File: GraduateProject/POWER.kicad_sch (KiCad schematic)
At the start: 24 parts, among them J2 Conn_01x04_Pin, U1 TLP181GB-S, U2 78L05G-AB3-R, U3 78L05G-AB3-R, U4 26V-15V L78L15ABUTR

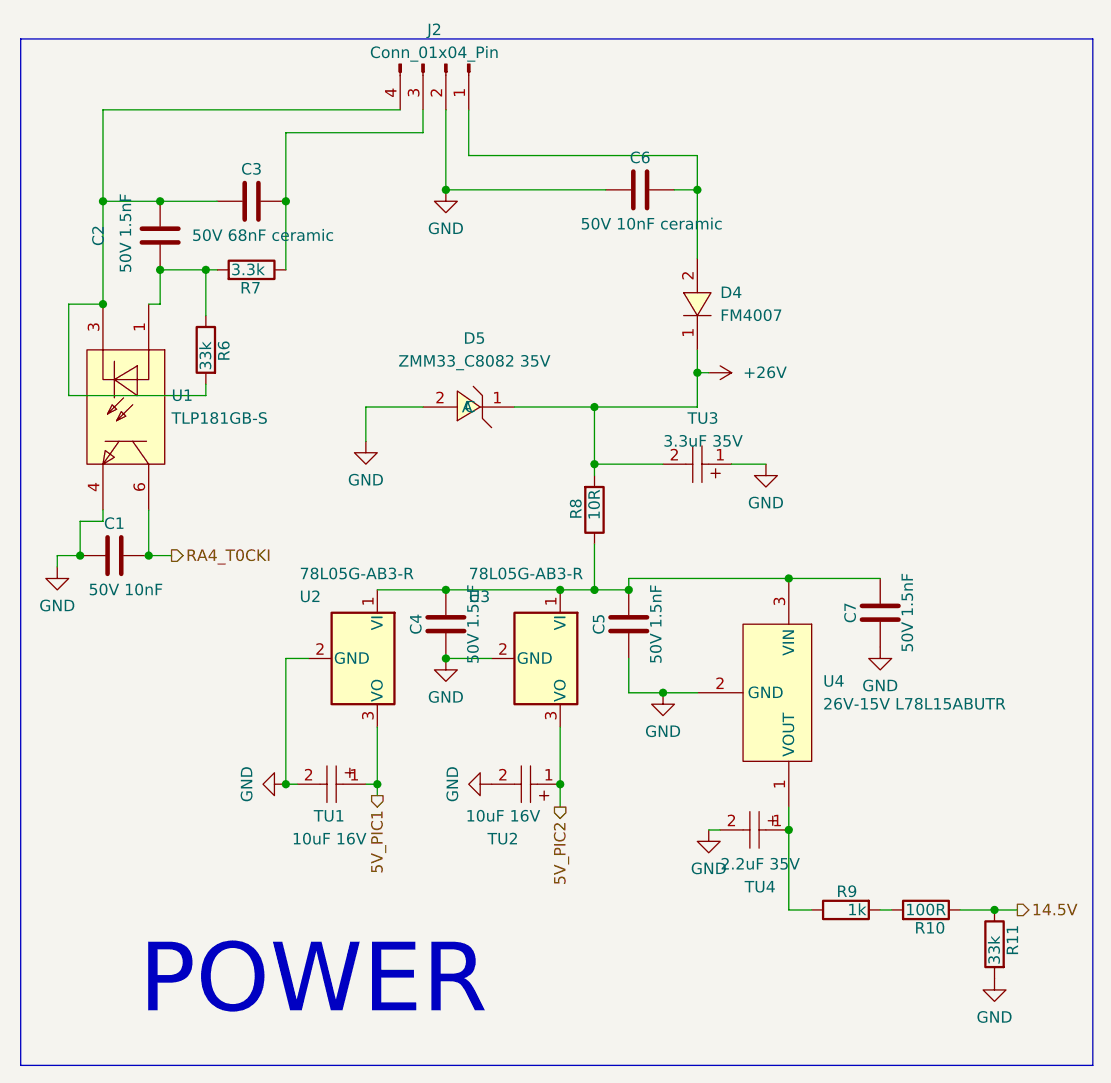
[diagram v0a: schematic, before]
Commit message: Add files via upload
17h37 11/9/2025
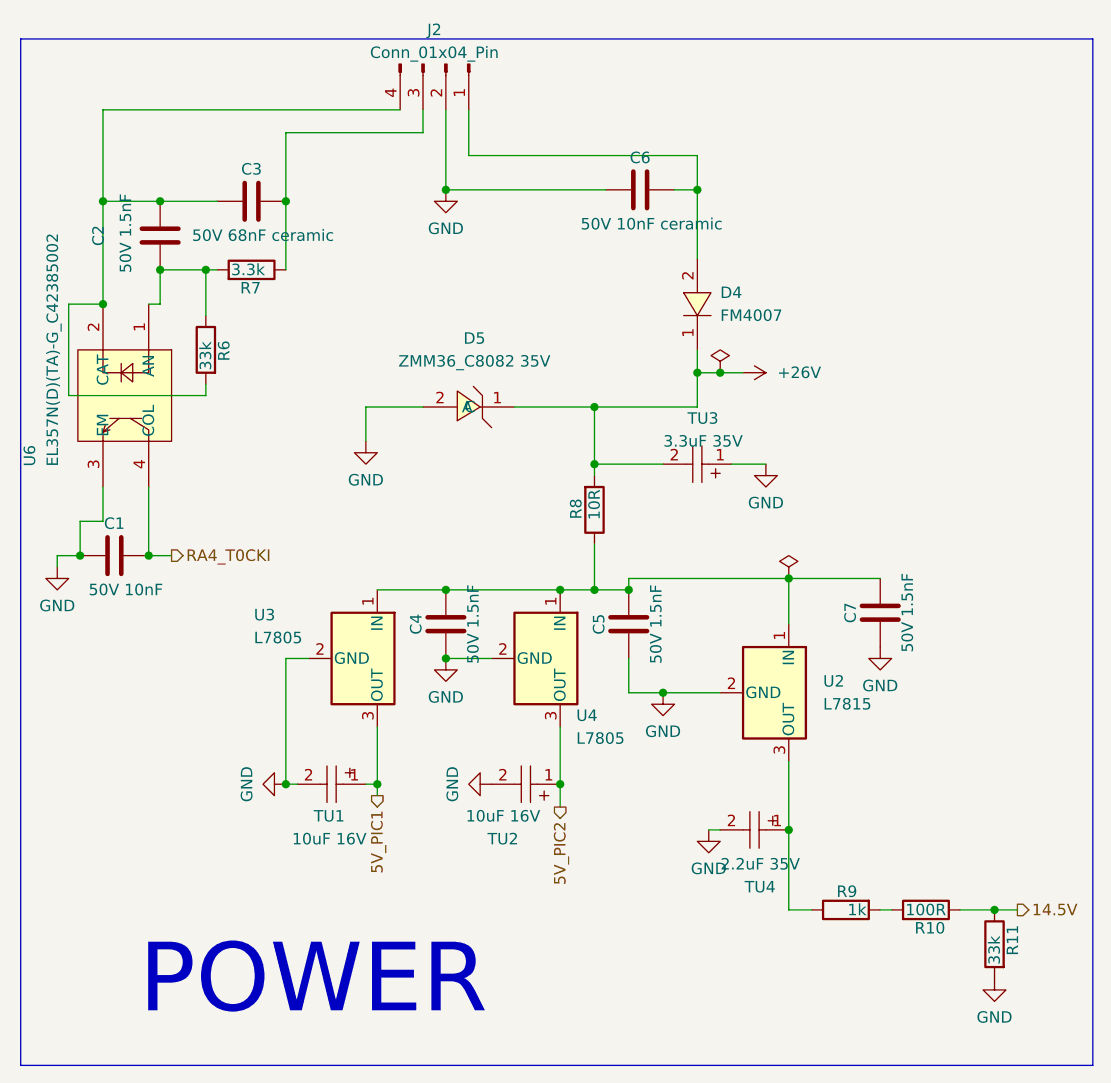
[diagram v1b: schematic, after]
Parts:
- removed U1: TLP181GB-S, easyeda2kicad:SOP-4_L3.7-W4.6-P2.54-LS7.0-TL, symbol easyeda2kicad:TLP181GB-S
- removed U2, U3: 78L05G-AB3-R, Package_TO_SOT_SMD:SOT-89-3, symbol Regulator_Linear:KA78M05_TO252
- removed U4: 26V-15V L78L15ABUTR, easyeda2kicad:SOT-89-3_L4.5-W2.5-P1.50-LS4.2-TL, symbol easyeda2kicad:L78L15ABUTR
- added U2: L7815, Package_TO_SOT_SMD:TO-263-2, symbol Regulator_Linear:L7815
- added U3, U4: L7805, Package_TO_SOT_SMD:TO-263-2, symbol Regulator_Linear:L7805
- added U6: EL357N(D)(TA)-G_C42385002, easyeda2kicad:SOP-4_L3.9-W4.4-P2.54-LS7.0-TL, symbol easyeda2kicad:EL357N(D)(TA)-G_C42385002
- D5: value ZMM33_C8082 35V -> ZMM36_C8082 35V
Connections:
- net 5V_PIC1: now also U3.3 (OUT)
- net 5V_PIC2: now also U4.3 (OUT)
- net GND: now also U2.2 (GND), U3.2 (GND), U4.2 (GND), U6.3 (EM)
- net RA4_T0CKI: now also U6.4 (COL)
- net at R9.1, TU4.1: now also U2.3 (OUT)
- net at C4.1, C5.1, C7.1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: now also U2.1 (IN), U3.1 (IN), U4.1 (IN)
- net at C2.2, R6.1, R7.2: now also U6.1 (AN)
- net at C2.1, C3.2, J2.4 (Pin_4)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: now also U6.2 (CAT)
